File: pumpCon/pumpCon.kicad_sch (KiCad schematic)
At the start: 86 parts, among them J1 USB_B_Micro, J2 Conn_01x03, J3 Conn_01x02, J4 Conn_01x03, J5 Conn_01x03, J6 Conn_01x02, J7 Conn_01x02, J8 Conn_01x03, J9 Conn_01x03, U1 W25Q16JVUXIQ, U2 RP2040, U3 AP2127K-ADJ, U4 TPS92200DxRXL, U5 MCP6001R, U6 AP63357Q, Y1 12Mhz

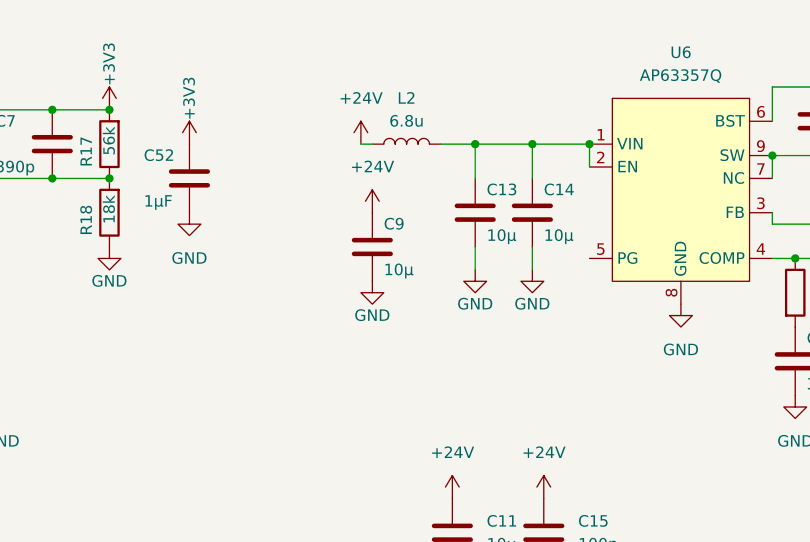
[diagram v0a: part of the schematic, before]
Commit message: wip
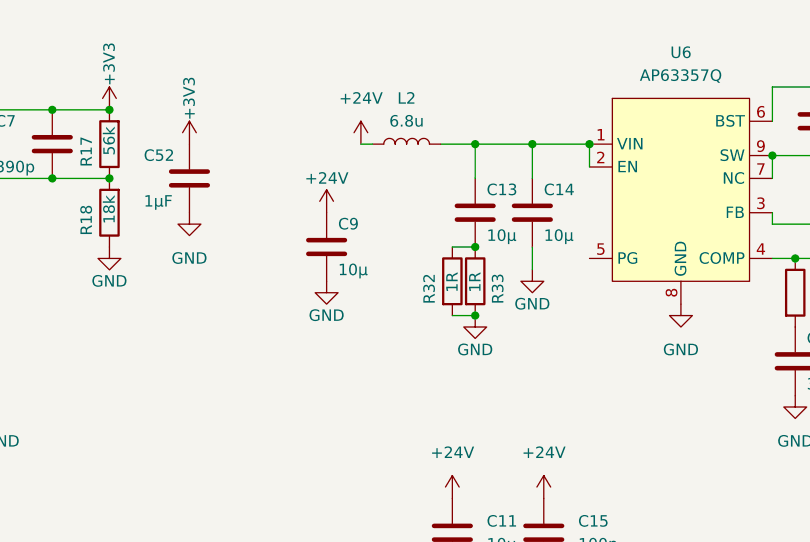
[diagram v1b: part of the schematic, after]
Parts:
- added R32, R33: 1R, Resistor_SMD:R_0603_1608Metric, symbol Device:R
- J6, J7: footprint Connector_PinSocket_2.54mm:PinSocket_1x02_P2.54mm_Vertical -> Connector_JST:JST_EH_B2B-EH-A_1x02_P2.50mm_Vertical
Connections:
- net GND: now also R32.2, R33.2; no longer C13.1
- new net: C13.1, R32.1, R33.1
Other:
- moved on the sheet: C9
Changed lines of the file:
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@@
   (junction (at 203.2 30.48) (diameter 0) (color 0 0 0 0)
   )
+  (junction (at 196.85 41.91) (diameter 0) (color 0 0 0 0)
+  )
   (junction (at 209.55 30.48) (diameter 0) (color 0 0 0 0)
   )
   (junction (at 229.87 31.75) (diameter 0) (color 0 0 0 0)
   )
+  (junction (at 196.85 49.53) (diameter 0) (color 0 0 0 0)
+  )
   (junction (at 250.19 31.75) (diameter 0) (color 0 0 0 0)
   )
@@
     (stroke (width 0) (type default) (color 0 0 0 0))
   )
+  (wire (pts (xy 194.31 41.91) (xy 196.85 41.91))
+    (stroke (width 0) (type default) (color 0 0 0 0))
+  )
   (wire (pts (xy 105.41 124.46) (xy 119.38 124.46))
     (stroke (width 0) (type default) (color 0 0 0 0))
@@
     (stroke (width 0) (type default) (color 0 0 0 0))
   )
-  (wire (pts (xy 196.85 44.45) (xy 196.85 41.91))
+  (wire (pts (xy 194.31 49.53) (xy 196.85 49.53))
     (stroke (width 0) (type default) (color 0 0 0 0))
   )
@@
       (effects (font (size 1.27 1.27)) (justify left))
     )
-    (property "Footprint" "Connector_PinSocket_2.54mm:PinSocket_1x02_P2.54mm_Vertical" (id 2) (at 205.74 91.44 0)
+    (property "Footprint" "Connector_JST:JST_EH_B2B-EH-A_1x02_P2.50mm_Vertical" (id 2) (at 205.74 91.44 0)
       (effects (font (size 1.27 1.27)) hide)
     )
@@
     (pin "1")
   )
-  (symbol (lib_id "power:+24V") (at 185.42 38.1 0) (unit 1)
-    (in_bom yes) (on_board yes) (fields_autoplaced)
-    (property "Reference" "#PWR0123" (id 0) (at 185.42 41.91 0)
+  (symbol (lib_id "power:+24V") (at 180.34 38.1 0) (unit 1)
+    (in_bom yes) (on_board yes)
+    (property "Reference" "#PWR0123" (id 0) (at 180.34 41.91 0)
       (effects (font (size 1.27 1.27)) hide)
     )
-    (property "Value" "+24V" (id 1) (at 185.42 33.02 0))
-    (property "Footprint" "" (id 2) (at 185.42 38.1 0)
+    (property "Value" "+24V" (id 1) (at 180.34 34.29 0))
+    (property "Footprint" "" (id 2) (at 180.34 38.1 0)
       (effects (font (size 1.27 1.27)) hide)
     )
-    (property "Datasheet" "" (id 3) (at 185.42 38.1 0)
+    (property "Datasheet" "" (id 3) (at 180.34 38.1 0)
       (effects (font (size 1.27 1.27)) hide)
     )
@@
       (effects (font (size 1.27 1.27)) (justify left))
     )
-    (property "Footprint" "Connector_PinSocket_2.54mm:PinSocket_1x02_P2.54mm_Vertical" (id 2) (at 199.39 128.27 0)
+    (property "Footprint" "Connector_JST:JST_EH_B2B-EH-A_1x02_P2.50mm_Vertical" (id 2) (at 199.39 128.27 0)
       (effects (font (size 1.27 1.27)) hide)
     )
@@
     (pin "1")
   )
-  (symbol (lib_id "Device:C") (at 185.42 41.91 180) (unit 1)
+  (symbol (lib_id "Device:C") (at 180.34 41.91 180) (unit 1)
     (in_bom yes) (on_board yes)
-    (property "Reference" "C9" (id 0) (at 186.69 39.37 0)
+    (property "Reference" "C9" (id 0) (at 181.61 39.37 0)
       (effects (font (size 1.27 1.27)) (justify right))
     )
-    (property "Value" "10µ" (id 1) (at 186.69 44.45 0)
+    (property "Value" "10µ" (id 1) (at 181.61 44.45 0)
       (effects (font (size 1.27 1.27)) (justify right))
     )
-    (property "Footprint" "Capacitor_SMD:C_1210_3225Metric" (id 2) (at 184.4548 38.1 0)
+    (property "Footprint" "Capacitor_SMD:C_1210_3225Metric" (id 2) (at 179.3748 38.1 0)
       (effects (font (size 1.27 1.27)) hide)
     )
-    (property "Datasheet" "~" (id 3) (at 185.42 41.91 0)
+    (property "Datasheet" "~" (id 3) (at 180.34 41.91 0)
       (effects (font (size 1.27 1.27)) hide)
     )
@@
     (pin "2")
   )
+  (symbol (lib_id "Device:R") (at 196.85 45.72 0) (unit 1)
+    (in_bom yes) (on_board yes)
+    (property "Reference" "R33" (id 0) (at 199.39 48.26 90)
+      (effects (font (size 1.27 1.27)) (justify left))
+    )
+    (property "Value" "1R" (id 1) (at 196.85 46.99 90)
+      (effects (font (size 1.27 1.27)) (justify left))
+    )
+    (property "Footprint" "Resistor_SMD:R_0603_1608Metric" (id 2) (at 195.072 45.72 90)
+      (effects (font (size 1.27 1.27)) hide)
+    )
+    (property "Datasheet" "~" (id 3) (at 196.85 45.72 0)
+      (effects (font (size 1.27 1.27)) hide)
+    )
+    (pin "1")
+    (pin "2")
+  )
   (symbol (lib_id "Device:C") (at 234.95 27.94 180) (unit 1)
     (in_bom yes) (on_board yes)
@@
     (pin "2")
   )
-  (symbol (lib_id "power:GND") (at 185.42 45.72 0) (unit 1)
+  (symbol (lib_id "power:GND") (at 180.34 45.72 0) (unit 1)
     (in_bom yes) (on_board yes)
-    (property "Reference" "#PWR0119" (id 0) (at 185.42 52.07 0)
+    (property "Reference" "#PWR0119" (id 0) (at 180.34 52.07 0)
       (effects (font (size 1.27 1.27)) hide)
     )
-    (property "Value" "GND" (id 1) (at 185.42 49.53 0))
-    (property "Footprint" "" (id 2) (at 185.42 45.72 0)
+    (property "Value" "GND" (id 1) (at 180.34 49.53 0))
+    (property "Footprint" "" (id 2) (at 180.34 45.72 0)
       (effects (font (size 1.27 1.27)) hide)
     )
-    (property "Datasheet" "" (id 3) (at 185.42 45.72 0)
+    (property "Datasheet" "" (id 3) (at 180.34 45.72 0)
       (effects (font (size 1.27 1.27)) hide)
     )
@@
     (pin "1")
   )
+  (symbol (lib_id "Device:R") (at 194.31 45.72 0) (unit 1)
+    (in_bom yes) (on_board yes)
+    (property "Reference" "R32" (id 0) (at 191.77 48.26 90)
+      (effects (font (size 1.27 1.27)) (justify left))
+    )
+    (property "Value" "1R" (id 1) (at 194.31 46.99 90)
+      (effects (font (size 1.27 1.27)) (justify left))
+    )
+    (property "Footprint" "Resistor_SMD:R_0603_1608Metric" (id 2) (at 192.532 45.72 90)
+      (effects (font (size 1.27 1.27)) hide)
+    )
+    (property "Datasheet" "~" (id 3) (at 194.31 45.72 0)
+      (effects (font (size 1.27 1.27)) hide)
+    )
+    (pin "1")
+    (pin "2")
+  )
   (symbol (lib_id "power:+3V3") (at 246.38 82.55 0) (unit 1)
     (in_bom yes) (on_board yes)
@@
     (pin "1")
   )
-  (symbol (lib_id "power:GND") (at 196.85 44.45 0) (unit 1)
+  (symbol (lib_id "power:GND") (at 196.85 49.53 0) (unit 1)
     (in_bom yes) (on_board yes)
-    (property "Reference" "#PWR0124" (id 0) (at 196.85 50.8 0)
+    (property "Reference" "#PWR0124" (id 0) (at 196.85 55.88 0)
       (effects (font (size 1.27 1.27)) hide)
     )
-    (property "Value" "GND" (id 1) (at 196.85 48.26 0))
-    (property "Footprint" "" (id 2) (at 196.85 44.45 0)
+    (property "Value" "GND" (id 1) (at 196.85 53.34 0))
+    (property "Footprint" "" (id 2) (at 196.85 49.53 0)
       (effects (font (size 1.27 1.27)) hide)
     )
-    (property "Datasheet" "" (id 3) (at 196.85 44.45 0)
+    (property "Datasheet" "" (id 3) (at 196.85 49.53 0)
       (effects (font (size 1.27 1.27)) hide)
     )
@@
     )
     (path "/571f6d5e-59b7-44e1-852d-cf47bc65ea21"
-      (reference "J6") (unit 1) (value "Conn_01x02") (footprint "Connector_PinSocket_2.54mm:PinSocket_1x02_P2.54mm_Vertical")
+      (reference "J6") (unit 1) (value "Conn_01x02") (footprint "Connector_JST:JST_EH_B2B-EH-A_1x02_P2.50mm_Vertical")
     )
     (path "/038f88d0-25cb-4cbc-9f1a-53363bad139d"
-      (reference "J7") (unit 1) (value "Conn_01x02") (footprint "Connector_PinSocket_2.54mm:PinSocket_1x02_P2.54mm_Vertical")
+      (reference "J7") (unit 1) (value "Conn_01x02") (footprint "Connector_JST:JST_EH_B2B-EH-A_1x02_P2.50mm_Vertical")
     )
     (path "/116b1d26-d7be-4274-a9fd-1e5101ff22f1"
@@
       (reference "R31") (unit 1) (value "1.1k") (footprint "Resistor_SMD:R_0603_1608Metric")
     )
+    (path "/d14c4765-591d-4cb7-8c13-bf02d74563c6"
+      (reference "R32") (unit 1) (value "1R") (footprint "Resistor_SMD:R_0603_1608Metric")
+    )
+    (path "/cd1a0824-5270-4dae-a15c-2109703f72e0"
+      (reference "R33") (unit 1) (value "1R") (footprint "Resistor_SMD:R_0603_1608Metric")
+    )
     (path "/c6c82006-26c7-4641-9e87-e0fdb5b42a77"
